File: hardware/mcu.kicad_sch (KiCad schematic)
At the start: 17 parts, among them J1 Micro_SD_Card, J3 USB_C_Receptacle_USB2.0_14P, Q1 Q_NPN_BEC, Q2 Q_NPN_BEC, U1 ESP32-S3-WROOM-1, U6 CH340G

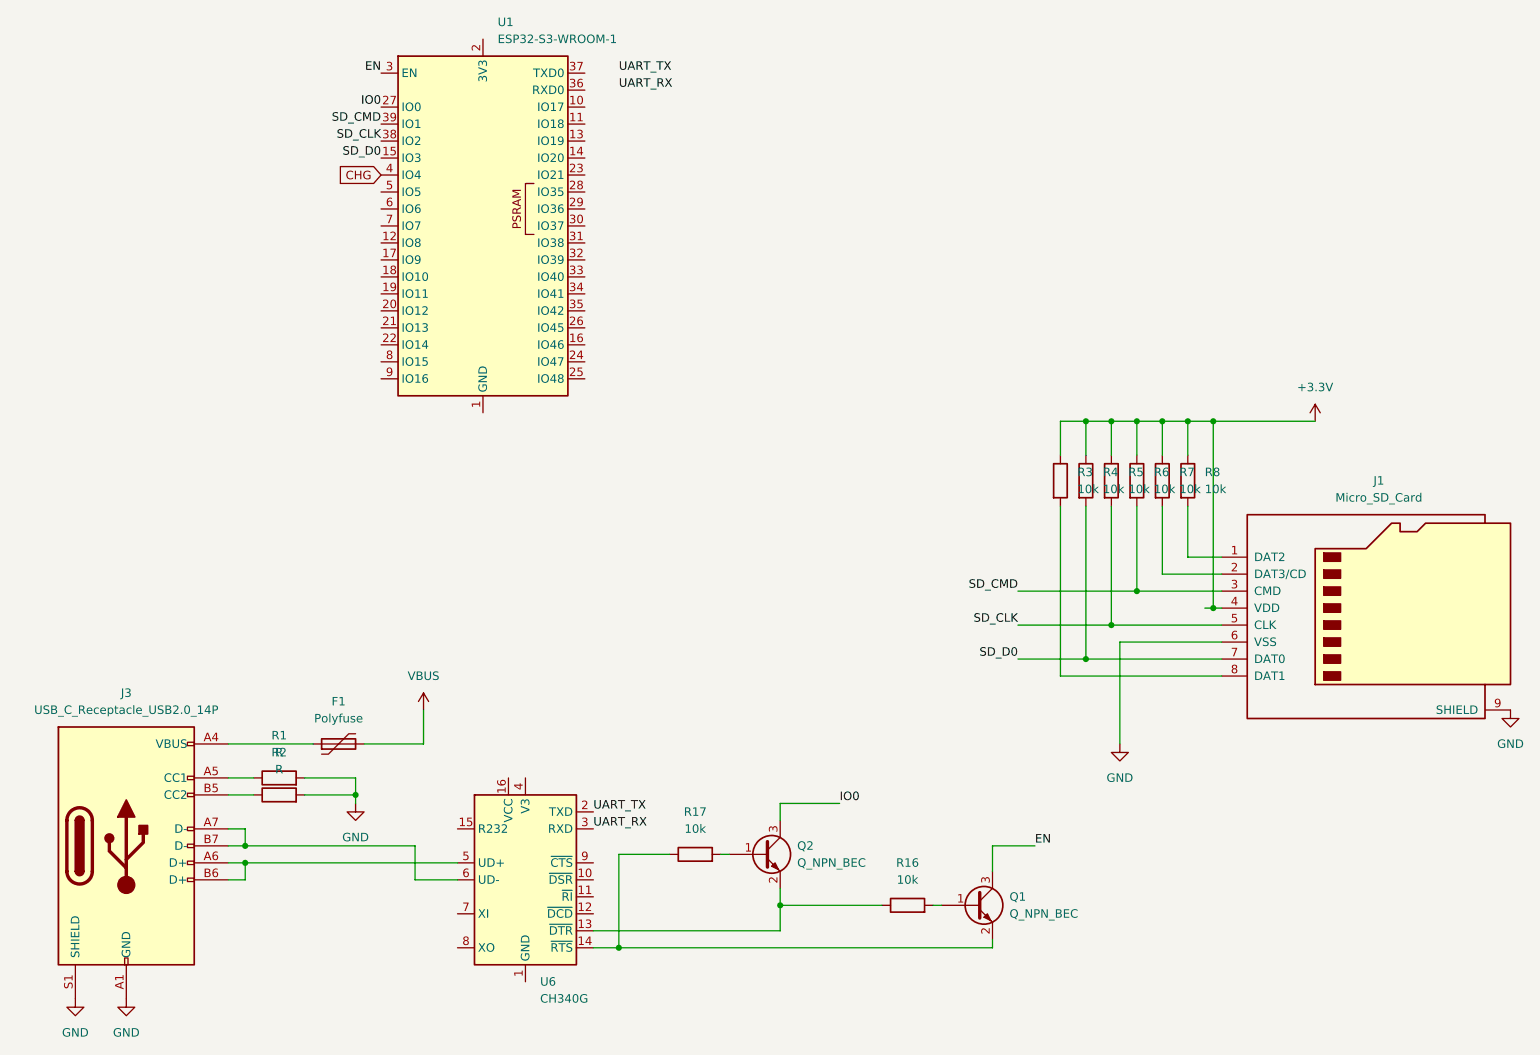
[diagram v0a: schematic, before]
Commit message: fix ch340
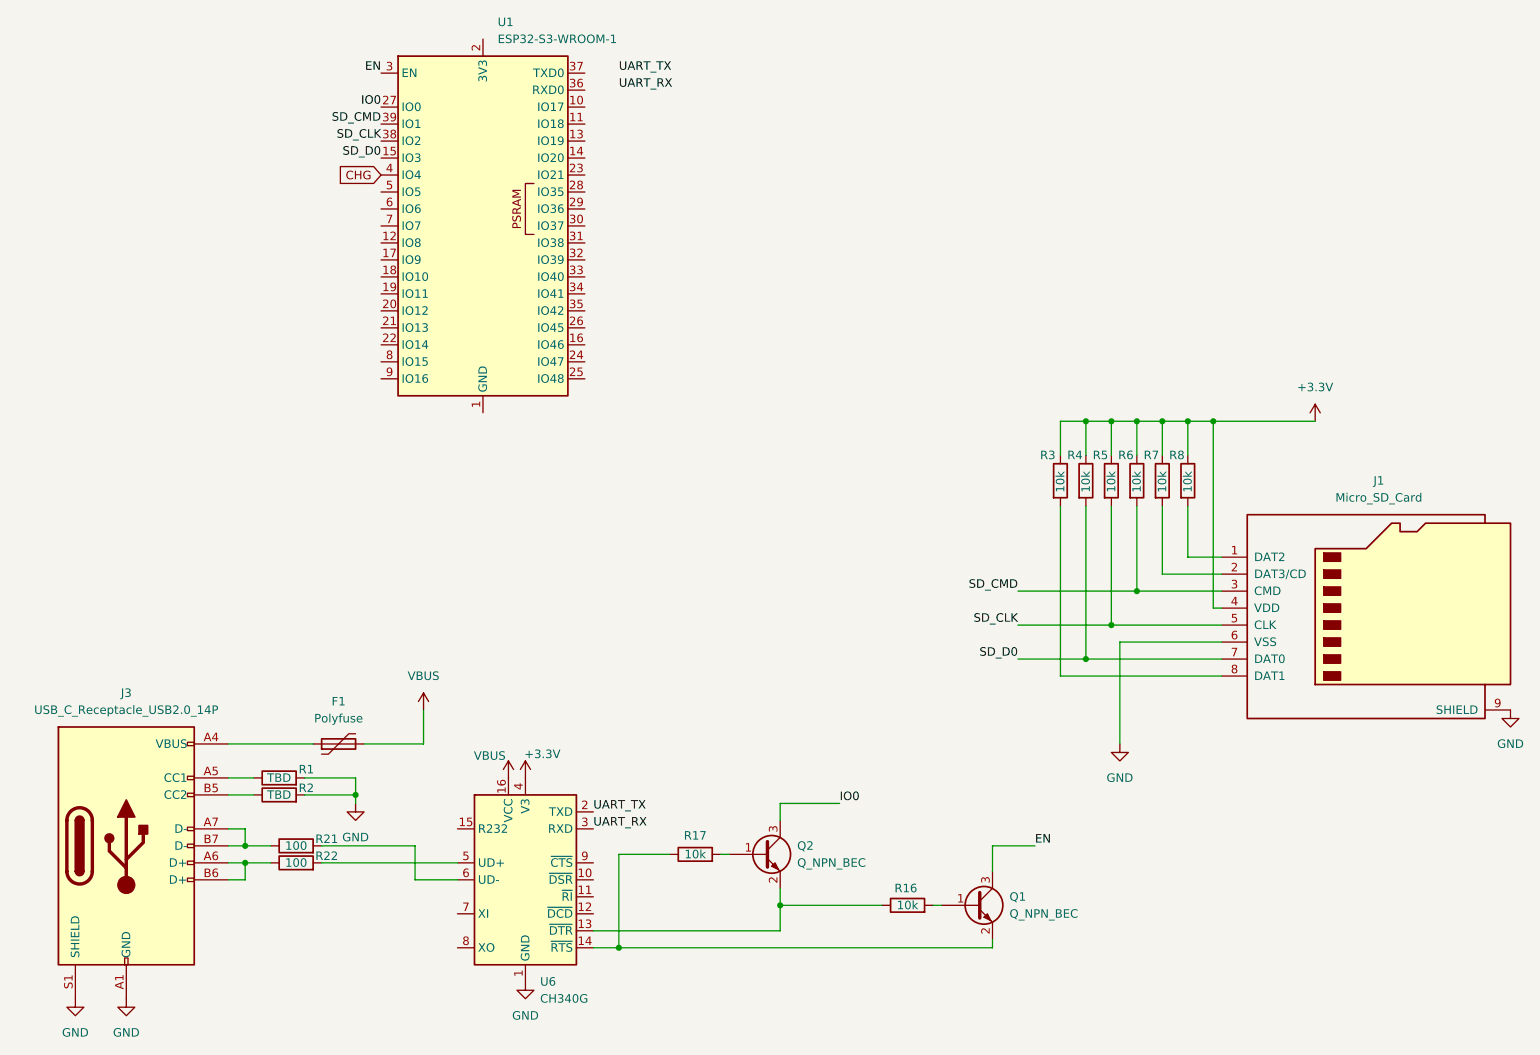
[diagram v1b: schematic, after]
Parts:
- added R21, R22: 100, Resistor_SMD:R_0201_0603Metric, symbol Device:R
- R1, R2: value R -> TBD
- U6: LCSC (none) -> C14267
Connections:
- net +3.3V: now also U6.4 (V3)
- net GND: now also U6.1 (GND)
- net VBUS: now also U6.16 (VCC)
- net at J3.A6 (D+), J3.B6 (D+): now also R22.1; no longer U6.5 (UD+)
- net at J3.A7 (D-), J3.B7 (D-): now also R21.1; no longer U6.6 (UD-)
- new net: R22.2, U6.5 (UD+)
- new net: R21.2, U6.6 (UD-)

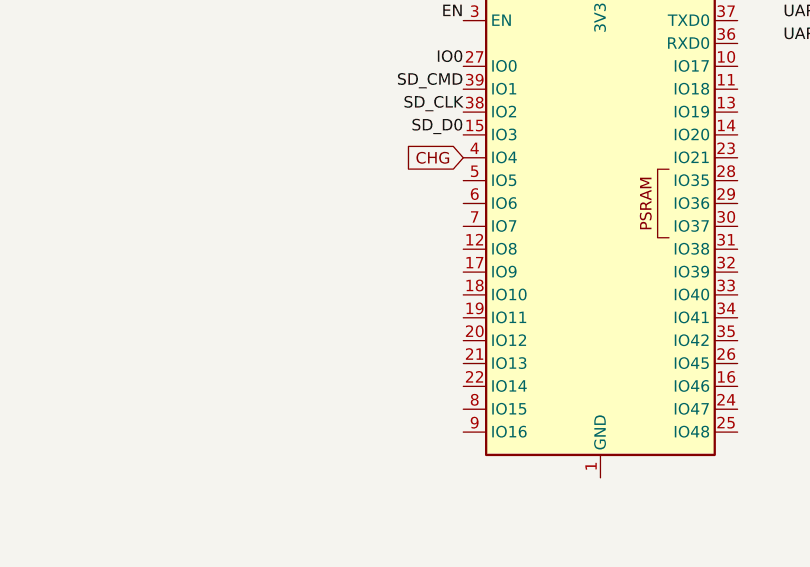
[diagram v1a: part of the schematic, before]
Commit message: keyboard schematic
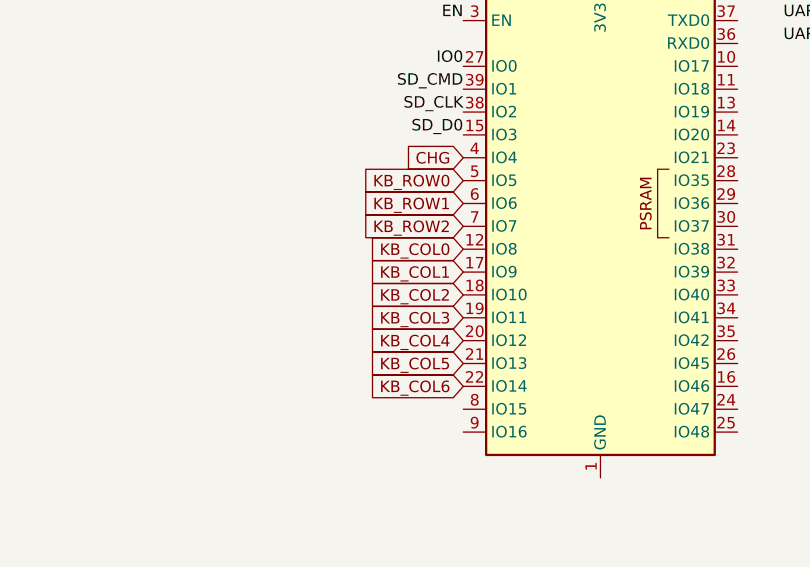
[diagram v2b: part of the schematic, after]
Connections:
- net KB_COL0: now reaches U1.12 (IO8)
- net KB_COL1: now reaches U1.17 (IO9)
- net KB_COL2: now reaches U1.18 (IO10)
- net KB_COL3: now reaches U1.19 (IO11)
- net KB_COL4: now reaches U1.20 (IO12)
- net KB_COL5: now reaches U1.21 (IO13)
- net KB_COL6: now reaches U1.22 (IO14)
- net KB_ROW0: now reaches U1.5 (IO5)
- net KB_ROW1: now reaches U1.6 (IO6)
- net KB_ROW2: now reaches U1.7 (IO7)
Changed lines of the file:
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@@
+		)
+	)
+	(global_label "KB_ROW0"
+		(shape input)
+		(at 71.12 60.96 180)
+		(fields_autoplaced yes)
+		(effects
+			(font
+				(size 1.27 1.27)
+			)
+			(justify right)
+		)
+		(property "Intersheetrefs" "${INTERSHEET_REFS}"
+			(at 59.3658 60.96 0)
+			(effects
+				(font
+					(size 1.27 1.27)
+				)
+				(justify right)
+				(hide yes)
+			)
+		)
+	)
+	(global_label "KB_COL0"
+		(shape input)
+		(at 71.12 68.58 180)
+		(fields_autoplaced yes)
+		(effects
+			(font
+				(size 1.27 1.27)
+			)
+			(justify right)
+		)
+		(property "Intersheetrefs" "${INTERSHEET_REFS}"
+			(at 59.7891 68.58 0)
+			(effects
+				(font
+					(size 1.27 1.27)
+				)
+				(justify right)
+				(hide yes)
+			)
+		)
+	)
+	(global_label "KB_ROW1"
+		(shape input)
+		(at 71.12 63.5 180)
+		(fields_autoplaced yes)
+		(effects
+			(font
+				(size 1.27 1.27)
+			)
+			(justify right)
+		)
+		(property "Intersheetrefs" "${INTERSHEET_REFS}"
+			(at 59.3658 63.5 0)
+			(effects
+				(font
+					(size 1.27 1.27)
+				)
+				(justify right)
+				(hide yes)
+			)
 		)
 	)
@@
 			(effects
 				(font
+					(size 1.27 1.27)
+				)
+				(justify right)
+				(hide yes)
+			)
+		)
+	)
+	(global_label "KB_COL1"
+		(shape input)
+		(at 71.12 71.12 180)
+		(fields_autoplaced yes)
+		(effects
+			(font
+				(size 1.27 1.27)
+			)
+			(justify right)
+		)
+		(property "Intersheetrefs" "${INTERSHEET_REFS}"
+			(at 59.7891 71.12 0)
+			(effects
+				(font
+					(size 1.27 1.27)
+				)
+				(justify right)
+				(hide yes)
+			)
+		)
+	)
+	(global_label "KB_COL4"
+		(shape input)
+		(at 71.12 78.74 180)
+		(fields_autoplaced yes)
+		(effects
+			(font
+				(size 1.27 1.27)
+			)
+			(justify right)
+		)
+		(property "Intersheetrefs" "${INTERSHEET_REFS}"
+			(at 59.7891 78.74 0)
+			(effects
+				(font
+					(size 1.27 1.27)
+				)
+				(justify right)
+				(hide yes)
+			)
+		)
+	)
+	(global_label "KB_COL2"
+		(shape input)
+		(at 71.12 73.66 180)
+		(fields_autoplaced yes)
+		(effects
+			(font
+				(size 1.27 1.27)
+			)
+			(justify right)
+		)
+		(property "Intersheetrefs" "${INTERSHEET_REFS}"
+			(at 59.7891 73.66 0)
+			(effects
+				(font
+					(size 1.27 1.27)
+				)
+				(justify right)
+				(hide yes)
+			)
+		)
+	)
+	(global_label "KB_COL5"
+		(shape input)
+		(at 71.12 81.28 180)
+		(fields_autoplaced yes)
+		(effects
+			(font
+				(size 1.27 1.27)
+			)
+			(justify right)
+		)
+		(property "Intersheetrefs" "${INTERSHEET_REFS}"
+			(at 59.7891 81.28 0)
+			(effects
+				(font
+					(size 1.27 1.27)
+				)
+				(justify right)
+				(hide yes)
+			)
+		)
+	)
+	(global_label "KB_COL6"
+		(shape input)
+		(at 71.12 83.82 180)
+		(fields_autoplaced yes)
+		(effects
+			(font
+				(size 1.27 1.27)
+			)
+			(justify right)
+		)
+		(property "Intersheetrefs" "${INTERSHEET_REFS}"
+			(at 59.7891 83.82 0)
+			(effects
+				(font
+					(size 1.27 1.27)
+				)
+				(justify right)
+				(hide yes)
+			)
+		)
+	)
+	(global_label "KB_ROW2"
+		(shape input)
+		(at 71.12 66.04 180)
+		(fields_autoplaced yes)
+		(effects
+			(font
+				(size 1.27 1.27)
+			)
+			(justify right)
+		)
+		(property "Intersheetrefs" "${INTERSHEET_REFS}"
+			(at 59.3658 66.04 0)
+			(effects
+				(font
+					(size 1.27 1.27)
+				)
+				(justify right)
+				(hide yes)
+			)
+		)
+	)
+	(global_label "KB_COL3"
+		(shape input)
+		(at 71.12 76.2 180)
+		(fields_autoplaced yes)
+		(effects
+			(font
+				(size 1.27 1.27)
+			)
+			(justify right)
+		)
+		(property "Intersheetrefs" "${INTERSHEET_REFS}"
+			(at 59.7891 76.2 0)
+			(effects
+				(font
